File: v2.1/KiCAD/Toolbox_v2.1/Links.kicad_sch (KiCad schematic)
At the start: 41 parts, among them J10 Links_1to3_OUT1, J11 Links_1to3_IN, J12 Links_1to3_OUT2, J13 Links_1to3_OUT3, J14 Links_2to2_IN1, J15 Links_2to2_IN2, J16 Links_2to2_OUT1, J17 Links_2to2_OUT2, J18 Links_3to1_IN1, J19 Links_3to1_IN2, J20 Links_3to1_OUT, J21 Links_3to1_IN3, U5 TL074, U6 TL074, U9 TL074

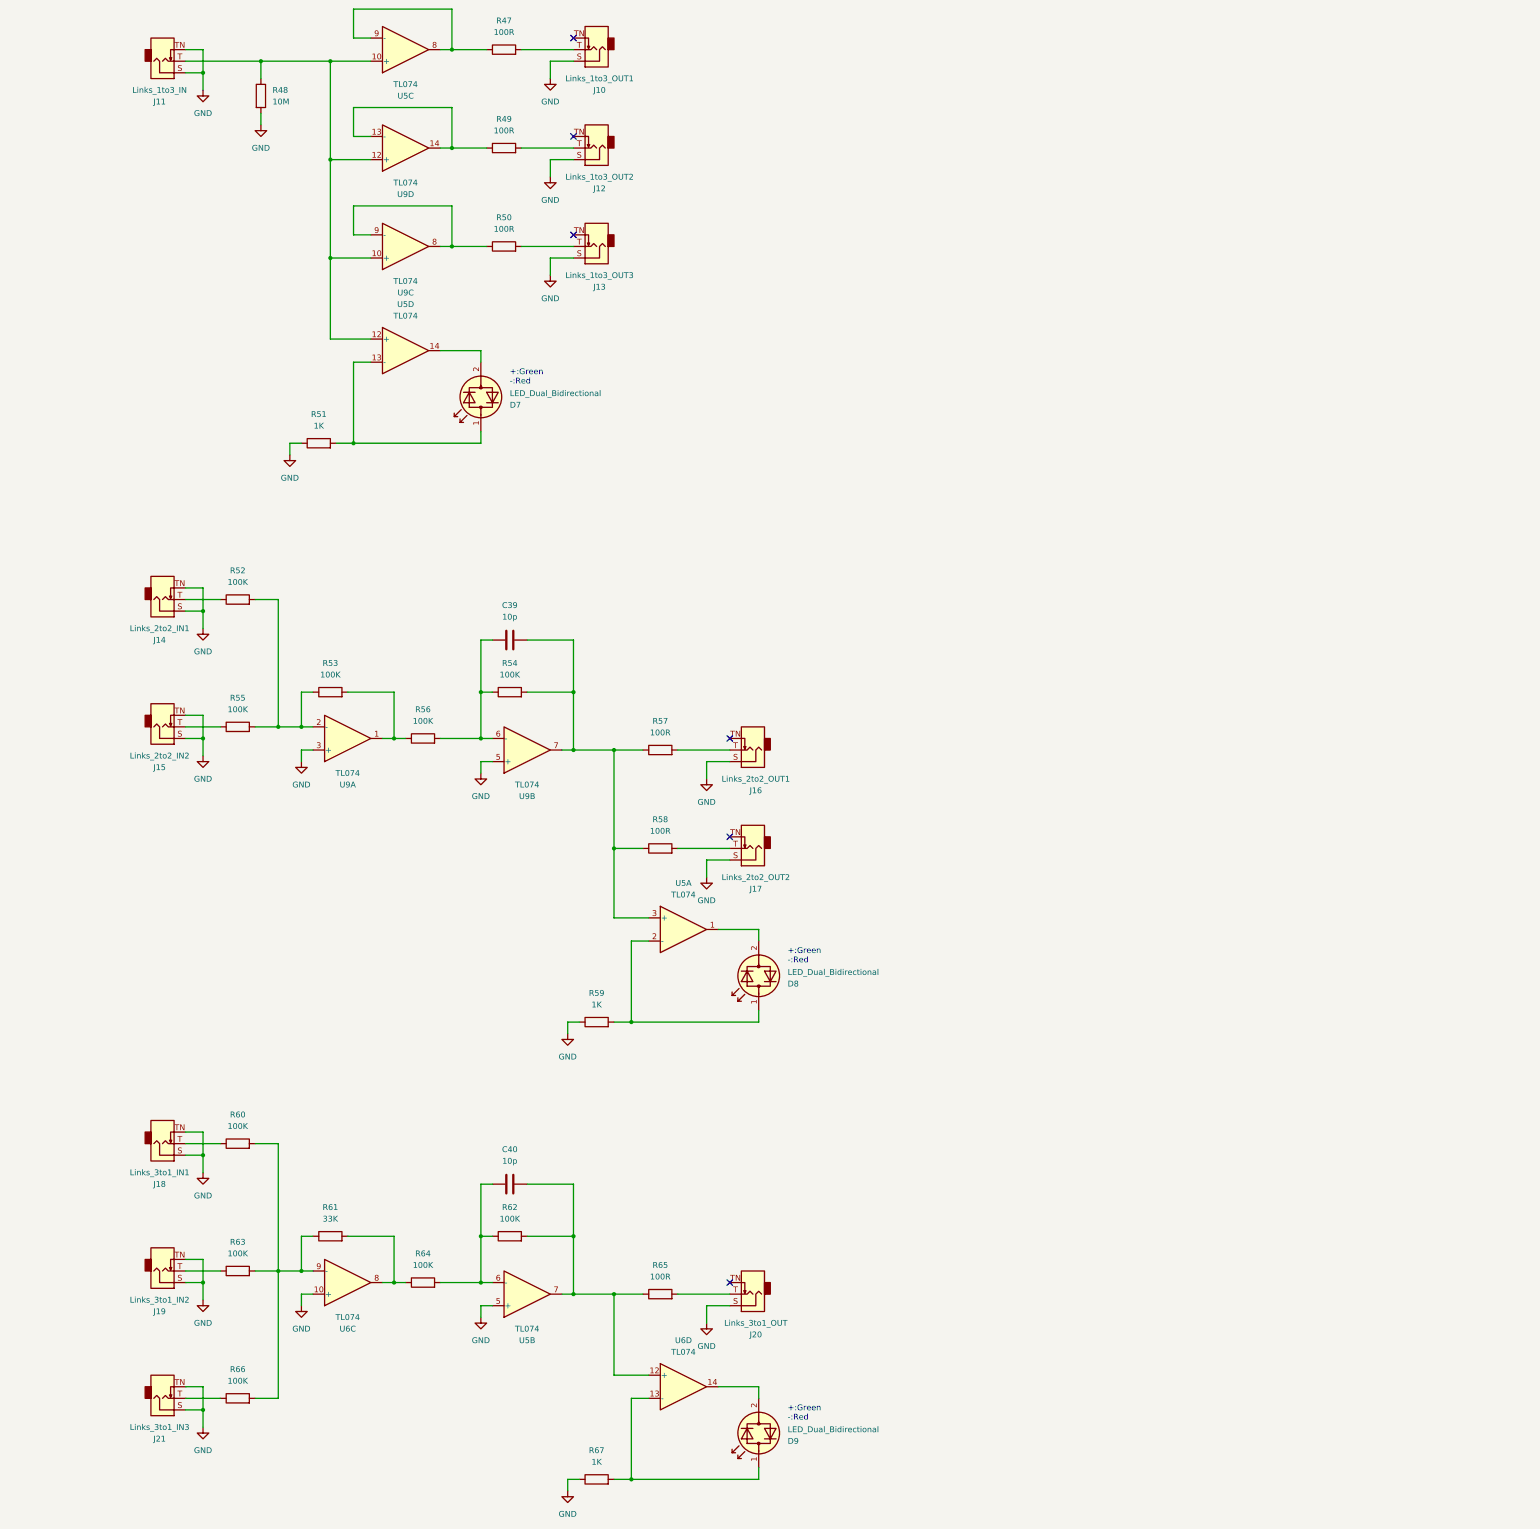
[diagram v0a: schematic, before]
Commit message: v2.1 Update
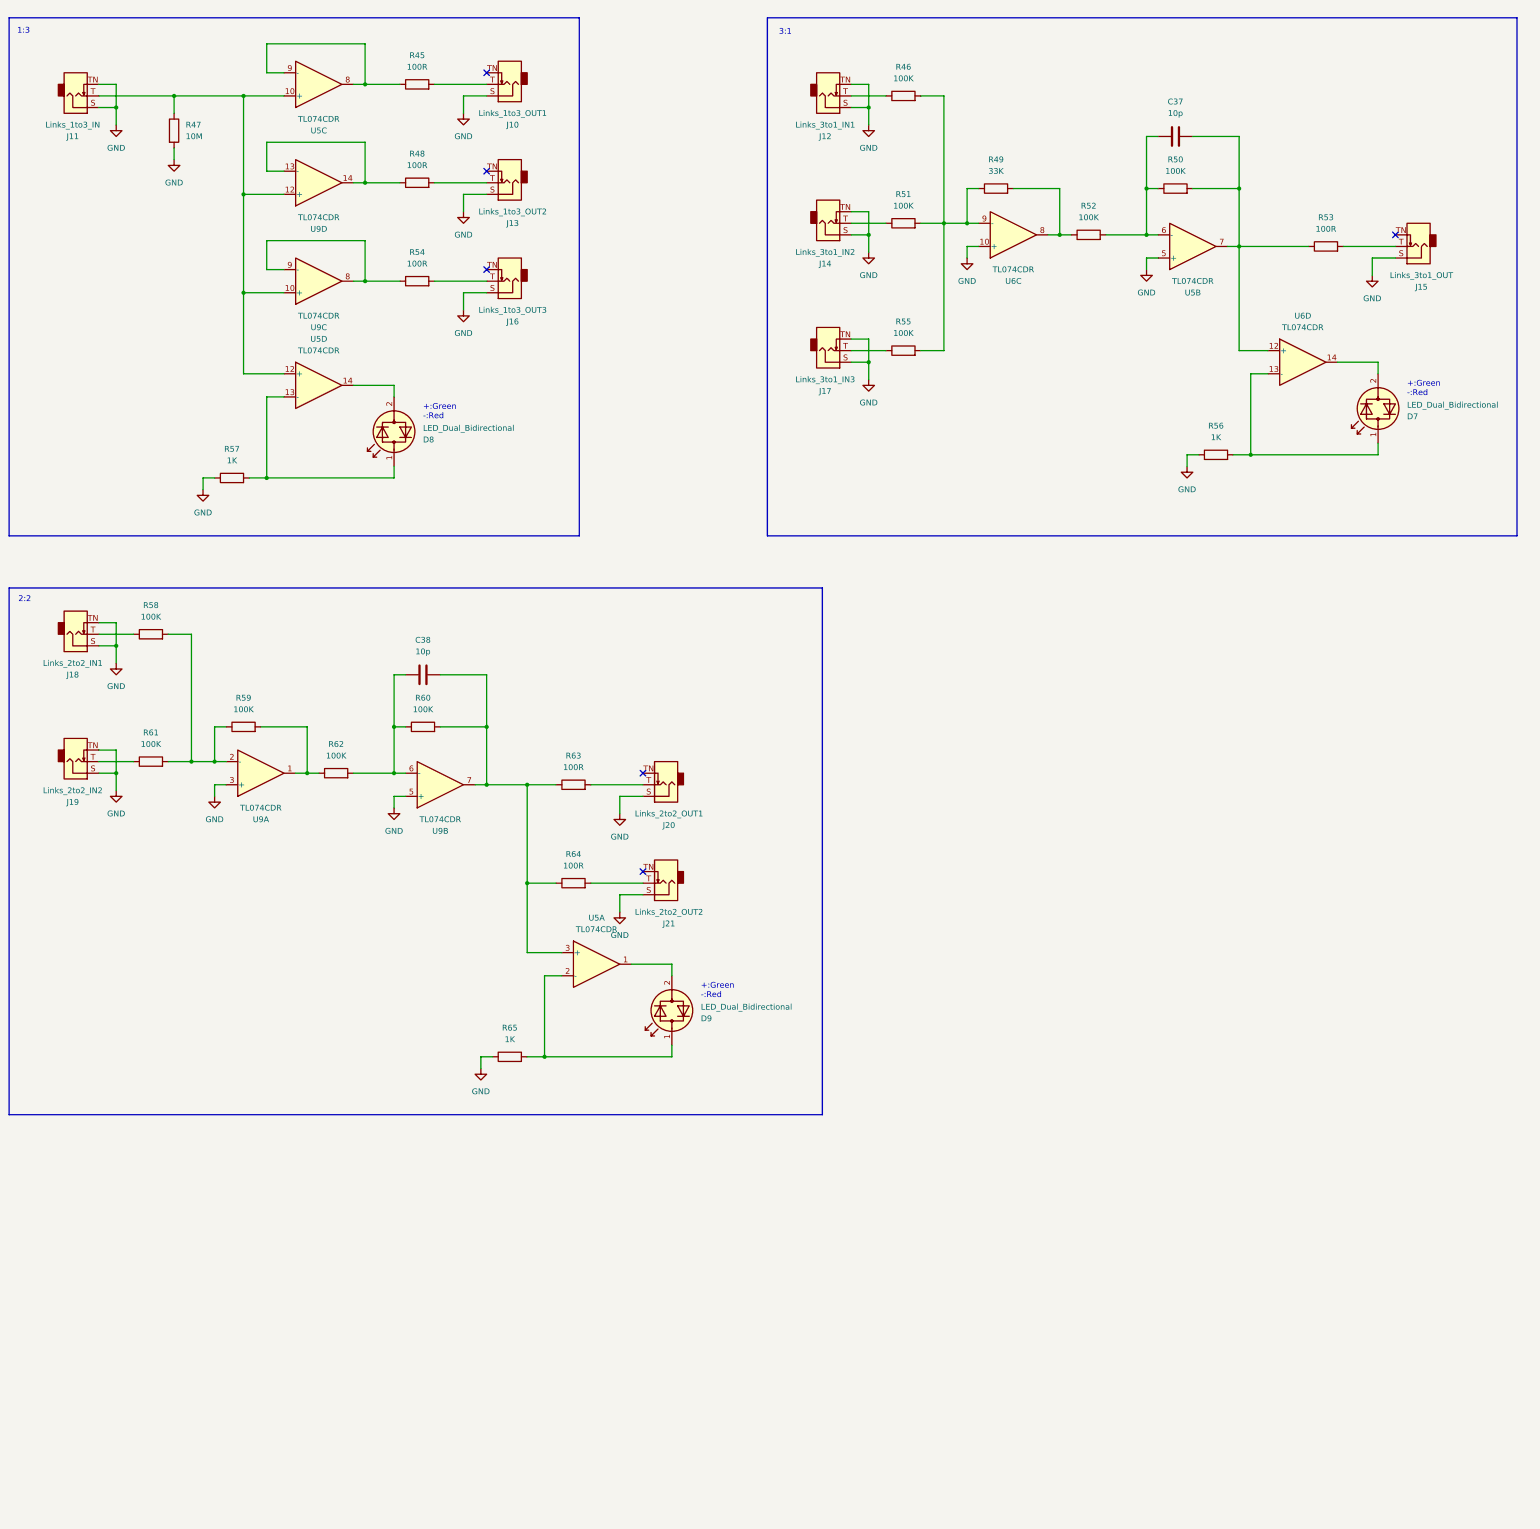
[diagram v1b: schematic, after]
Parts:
- U5, U6, U9: value TL074 -> TL074CDR; footprint Package_SO:TSSOP-14_4.4x5mm_P0.65mm -> Package_SO:SOIC-14_3.9x8.7mm_P1.27mm; LCSC C4370424 -> C12594
- renumbered C40 to C37, C39 to C38, D9 to D7, D7 to D8, D8 to D9, J18 to J12, J12 to J13, J19 to J14, J20 to J15, J13 to J16, J21 to J17, J14 to J18, J15 to J19, J16 to J20, J17 to J21, R47 to R45, R60 to R46, R48 to R47, R49 to R48, R61 to R49, R62 to R50, R63 to R51, R64 to R52, R65 to R53, R50 to R54, R66 to R55, R67 to R56, R51 to R57, R52 to R58, R53 to R59, R54 to R60, R55 to R61, R56 to R62, R57 to R63, R58 to R64, R59 to R65
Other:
- note added: "1:3"
- note added: "2:2"
- note added: "3:1"
- moved on the sheet: C37, C38, D7, D8, D9, J10, J11, J12, J13, J14, J15, J16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
